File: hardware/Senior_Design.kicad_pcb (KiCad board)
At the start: 4 copper layers, 111.5 x 73.6 mm, 147 parts, among them J101 Conn_ARM_JTAG_SWD_10, J201 54-00125, J202 Conn_01x03, J301 Conn_ARM_JTAG_SWD_10, J501 2305018-2, J601 J0011D21BNL, Q201 CSD87503Q3E, Q202 Q_NMOS, Q203 CSD87503Q3E, SW101 SW_Push, SW201 SW_Push, SW301 SW_Push, U101 EFR32FG28A122F1024GM48-A, U201 BQ25798RQMR, U202 TPS63020DSJR, U301 BDE-MB1352P71UA32, U401 TPS613222ADBVR, U402 BME688, U403 USBLC6-2P6, U501 CP2102N-A02-GQFN20, U502 CDSOT236-0504C, U601 W5500, Y101 LF_Crystal, Y102 ECS-390-CDX-1932, Y601 ECS-250-18-5PX-F-TR

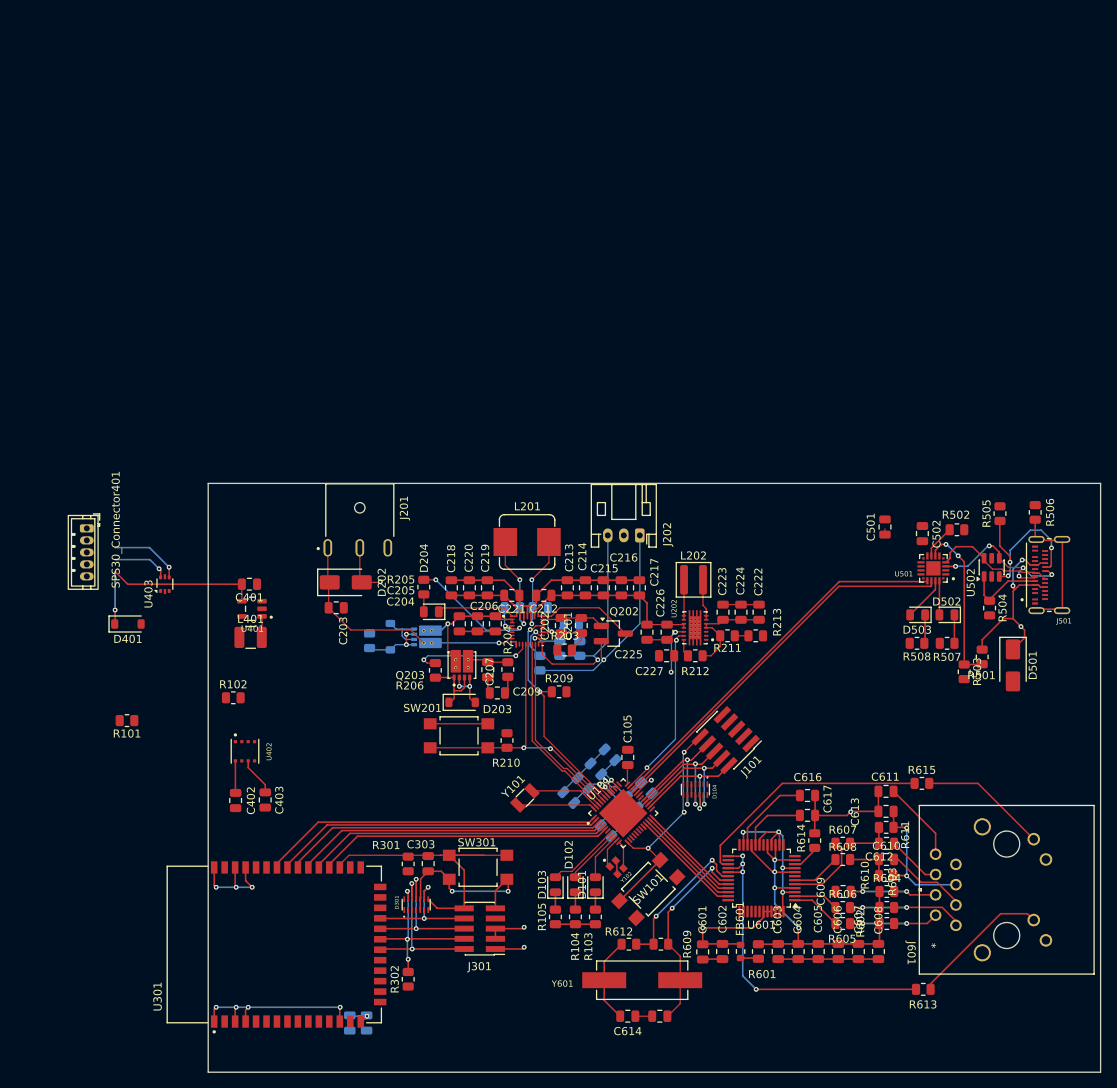
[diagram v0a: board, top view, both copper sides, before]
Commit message: Power Layout WIP
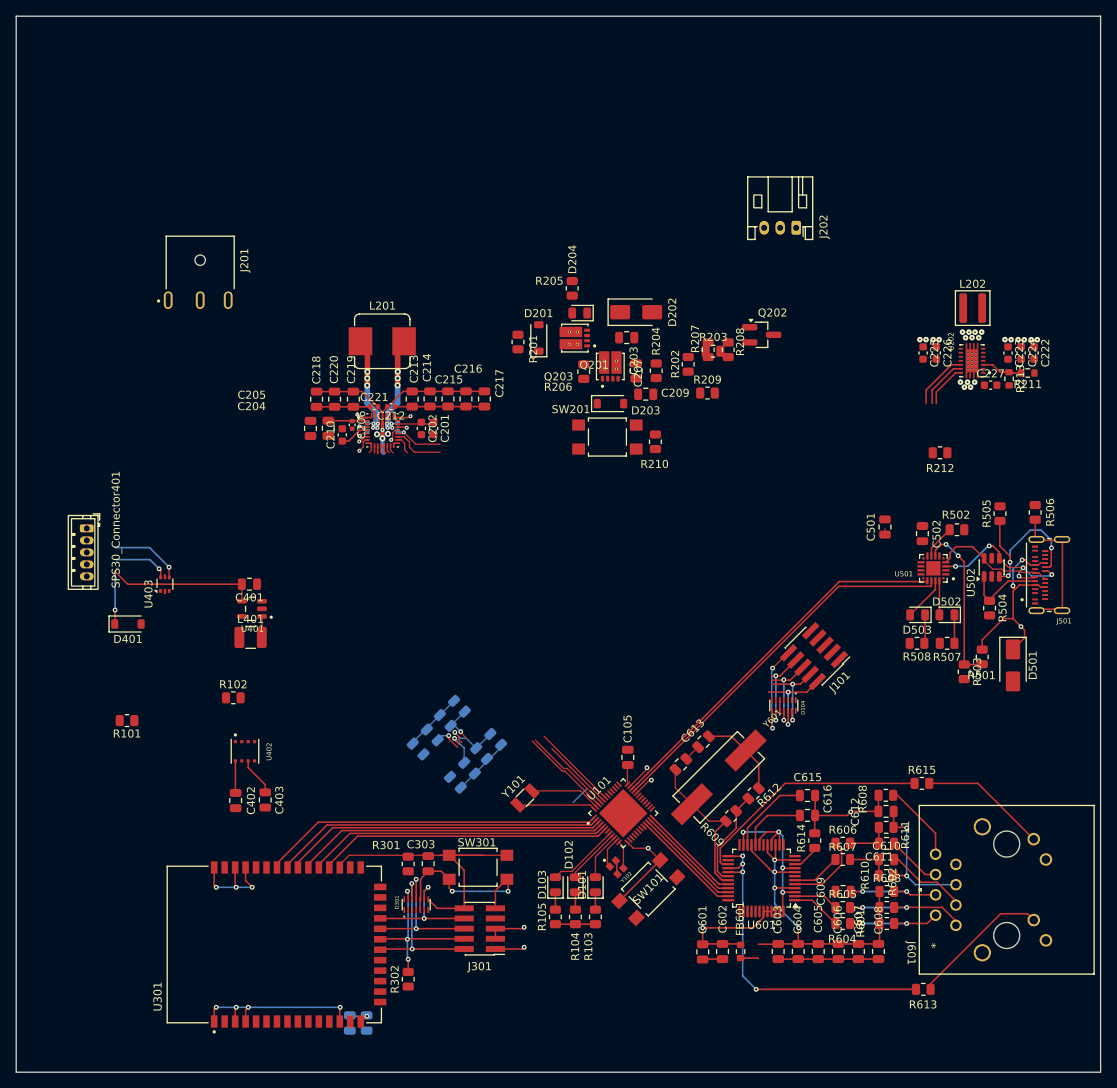
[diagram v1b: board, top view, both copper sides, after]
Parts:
- removed the C611 at (56.7, -14.1)
- C201, C202, C222, C223, C224, C225, C226, C227: footprint Capacitor_SMD:C_0805_2012Metric -> Capacitor_SMD:C_0603_1608Metric
- C206, C208, C211, C212, C221: footprint Capacitor_SMD:C_0805_2012Metric -> Capacitor_SMD:C_0402_1005Metric
- C210: footprint Capacitor_SMD:C_0805_2012Metric -> Capacitor_SMD:C_0603_1608Metric; moved to F.Cu
- D201, Q201, R201, R202, R207, R208: moved to F.Cu
- R211, R213: footprint Resistor_SMD:R_0805_2012Metric -> Resistor_SMD:R_0603_1608Metric
- moved C227 52.8 mm to (69.8, -64.9), turned to 0 degrees
- moved R211 49.9 mm to (74.4, -66.4), turned to 180 degrees
- moved C203 49.6 mm to (24.3, -70.8)
- moved D202 49.6 mm to (25.5, -74.0)
- moved C225 49.1 mm to (61.4, -68.9)
- moved L202 48.7 mm to (67.6, -74.5)
- moved C226 48.5 mm to (63.0, -68.9)
- moved C223 48.1 mm to (72.0, -68.9)
- moved U202 48.1 mm to (67.5, -67.9)
- moved C224 47.7 mm to (73.6, -68.9)
- moved C222 47.2 mm to (75.2, -68.9)
- moved R213 45.1 mm to (72.1, -65.7), turned to -90 degrees
- moved J202 43.1 mm to (45.5, -84.5)
- moved Q203 41.7 mm to (22.3, -67.2)
- moved R204 41.7 mm to (28.0, -66.7)
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- renumbered C612 to C611, C613 to C612, C614 to C613, C615 to C614, C616 to C615, C617 to C616, R602 to R601, R603 to R602, R604 to R603, R605 to R604, R606 to R605, R607 to R606, R608 to R607, R601 to R608
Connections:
- FB601 pad 2: Net-(FB601-Pad2) -> +3.3VA
- J601 pad 8: Net-(C611-Pad1) (its old number) -> Net-(J601-Pad8)
- R608 pad 1: +3.3VA -> Net-(J601-Pad8)
- R608 pad 2: Net-(FB601-Pad2) -> GND
- U202 pad 16: GND -> (no net)
- U202 pad 17: GND -> (no net)
- U202 pad 18: GND -> (no net)
- U202 pad 19: GND -> (no net)
- U202 pad 20: GND -> (no net)
- U202 pad 21: GND -> (no net)
- U202 pad 22: GND -> (no net)
- U202 pad 23: GND -> (no net)
- U202 pad 24: GND -> (no net)
- U202 pad 25: GND -> (no net)
- U202 pad 26: GND -> (no net)
- U202 pad 27: GND -> (no net)
- U202 pad 28: GND -> (no net)
- U202 pad 29: GND -> (no net)
- U202 pad 30: GND -> (no net)
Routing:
- net GND: track 211.9 -> 179.6 mm, vias 17 -> 42
- net /BMS/TS: track 30.0 -> 0.00 mm, vias 1 -> 0
- net /BMS/VAC2: track 31.7 -> 1.94 mm
- net Net-(J202-Pin_1): track 28.4 -> 0.00 mm, vias 1 -> 0
- net /BMS/QON: track 37.4 -> 10.0 mm, vias 2 -> 0
- net /BMS/BQ_INT: track 28.4 -> 12.0 mm, vias 2 -> 1
- net /BMS/REGN: track 22.2 -> 6.14 mm, vias 3 -> 0
- net /BMS/ACDRV1: track 15.1 -> 0.96 mm, vias 2 -> 0
- net +3.3V: track 36.8 -> 23.3 mm
- net /BMS/PS_SYNC: track 22.3 -> 9.69 mm, vias 2 -> 1
- net Net-(C204-Pad1): track 16.8 -> 4.89 mm, vias 1 -> 0
- net /BME 688 and SPS30/SCL: track 23.7 -> 12.6 mm
- net /BME 688 and SPS30/SDA: track 23.5 -> 12.5 mm
- net /BMS/SYS: track 23.6 -> 13.0 mm
- net Net-(Q202-G): track 12.1 -> 1.71 mm, vias 0 -> 1
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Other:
- board size 111.5 x 73.6 mm -> 135.6 x 132 mm
